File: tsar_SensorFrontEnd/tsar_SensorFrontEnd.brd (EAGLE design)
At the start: 128.5 x 85.1 mm, 217 parts, among them U1 ADS8344N, U2 ADS8344N

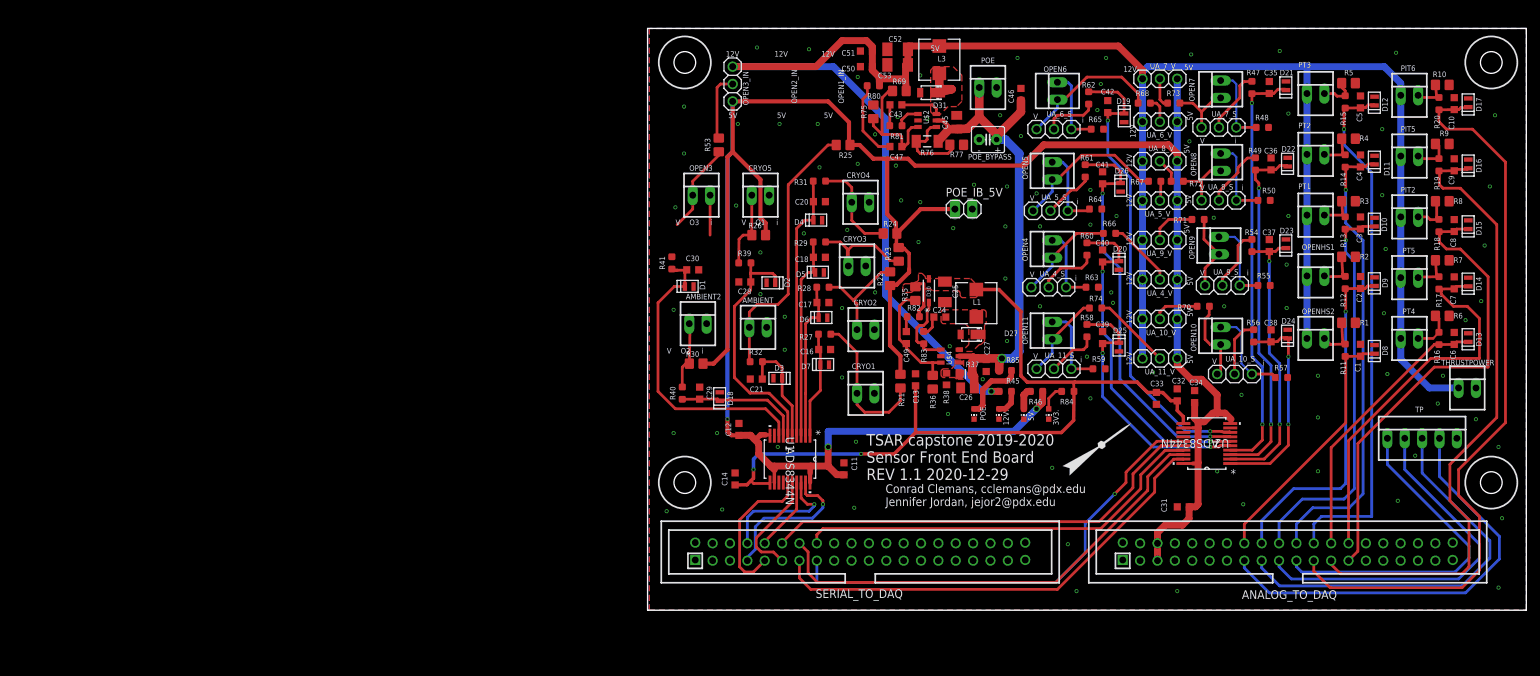
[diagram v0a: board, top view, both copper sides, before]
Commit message: POE, SFE changes
POE: added gnd vias and text info
SFE: moved to mar dxf outline. removed unallocated lines and added valve position sensor pinout. updated attributes. the board is currently unrouted.
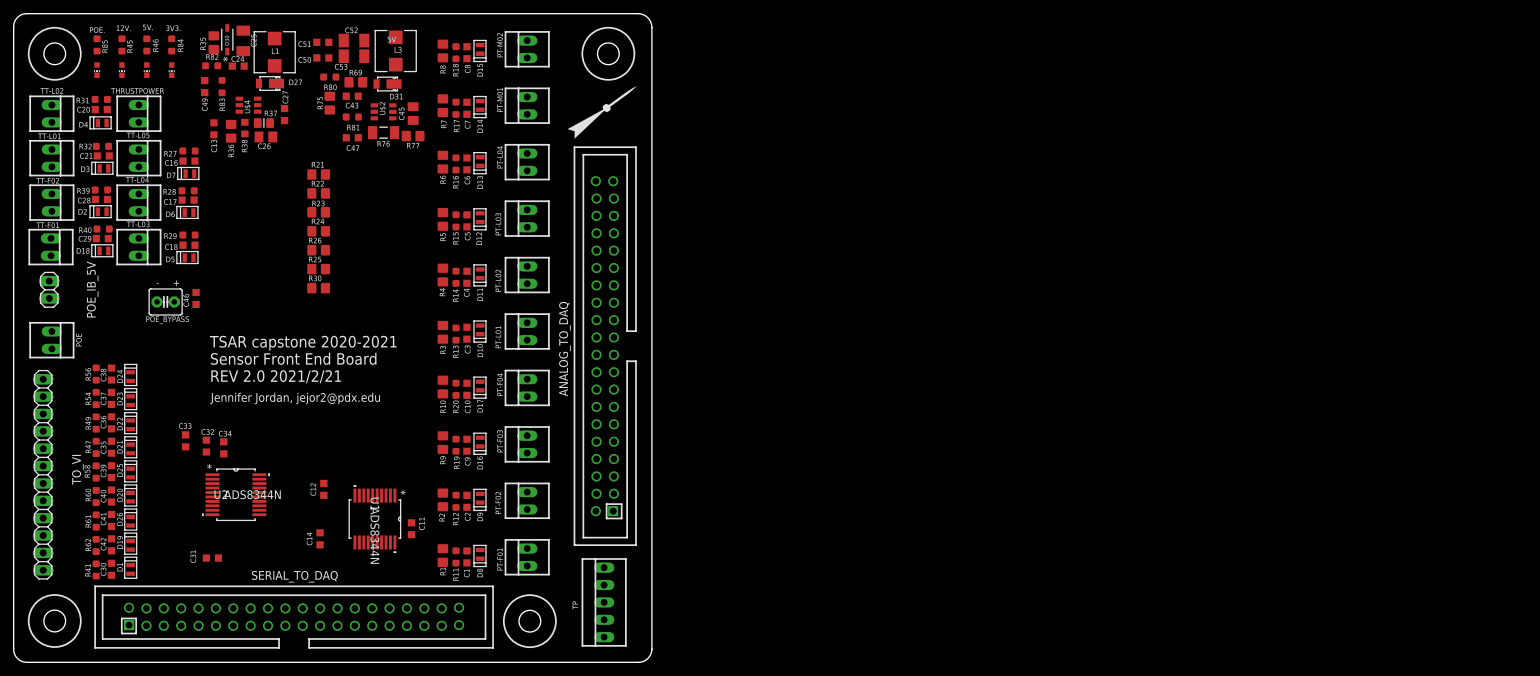
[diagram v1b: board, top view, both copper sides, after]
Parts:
- removed AMBIENT, AMBIENT2, CRYO1, CRYO2, CRYO3, CRYO4, CRYO5, OPEN10, OPEN3, OPEN7, OPEN8, OPEN9, OPENHS1, OPENHS2, PIT2, PIT5, PIT6, PT1, PT2, PT3, PT4, PT5: 22-23-2021, con-molex:22-23-2021
- removed JP3, UA_10_S, UA_10_V, UA_11_S, UA_11_V, UA_4_S, UA_4_V, UA_5_S, UA_5_V, UA_6_S, UA_6_V, UA_7_S, UA_7_V, UA_8_S, UA_8_V, UA_9_S, UA_9_V: (no value), adafruit:1X03
- removed OPEN11, OPEN4, OPEN5, OPEN6: (no value), con-molex:22-23-2021
- removed R48, R50, R55, R57, R59, R63, R64, R65, R66, R67, R68, R70, R71, R72, R73, R74: NP, oresat-rcl:.0603-A-NOSILK
- removed R53: NP, oresat-rcl:.0805-A-NOSILK
- added PT-F01, PT-F02, PT-F03, PT-F04, PT-L01, PT-L02, PT-L03, PT-L04, PT-M01, PT-M02, TT-F01, TT-F02, TT-L01, TT-L02, TT-L03, TT-L04, TT-L05: 22-23-2021, con-molex:22-23-2021
- added TO_VI: (no value), pinhead:1X12
- moved THRUSTPOWER 198.4 mm to (18.3, 80.2), turned to 270 degrees
- moved D21 177.3 mm to (17.0, 31.2), turned to 90 degrees
- moved C35 177.3 mm to (14.3, 31.5), turned to 270 degrees
- moved R47 177.0 mm to (12.1, 31.4), turned to 270 degrees
- moved C36 173.8 mm to (14.3, 35.0), turned to 270 degrees
- moved D22 173.7 mm to (17.0, 34.7), turned to 90 degrees
- moved R49 173.7 mm to (12.1, 35.0), turned to 270 degrees
- moved C37 170.8 mm to (14.3, 38.6), turned to 270 degrees
- moved D23 170.7 mm to (17.0, 38.3), turned to 90 degrees
- moved R54 170.5 mm to (12.1, 38.6), turned to 270 degrees
- moved C38 169.7 mm to (14.3, 42.2), turned to 270 degrees
- moved D24 169.6 mm to (17.0, 41.8), turned to 90 degrees
- moved R56 169.4 mm to (12.1, 42.2), turned to 270 degrees
- moved R62 159.2 mm to (12.1, 17.1)
- moved C42 159.2 mm to (14.3, 17.2), turned to 270 degrees
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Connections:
- removed net N$33: OPEN3.1, R41.2, R53.1
- removed net N$36: JP3.2, R53.2
- removed net N$55: R68.2, UA_6_V.2
- removed net N$57: R67.2, UA_5_V.2
- removed net N$58: R66.2, UA_4_V.2
- removed net N$59: OPEN4.2, R63.2, UA_4_S.3
- removed net N$60: OPEN5.2, R64.2, UA_5_S.3
- removed net N$61: OPEN6.2, R65.2, UA_6_S.3
- removed net N$62: OPEN6.1, R68.1, UA_6_S.1
- removed net N$63: OPEN5.1, R67.1, UA_5_S.1
- removed net N$64: OPEN4.1, R66.1, UA_4_S.1
- removed net N$65: OPEN7.2, R48.2, UA_7_S.3
- removed net N$66: OPEN7.1, R73.1, UA_7_S.1
- removed net N$67: R47.2, UA_7_S.2
- removed net N$68: R60.2, UA_4_S.2
- removed net N$69: R61.2, UA_5_S.2
- removed net N$70: R62.2, UA_6_S.2
- removed net N$71: OPEN8.2, R50.2, UA_8_S.3
- removed net N$72: OPEN8.1, R72.1, UA_8_S.1
- removed net N$73: R49.2, UA_8_S.2
- removed net N$74: OPEN9.2, R55.2, UA_9_S.3
- removed net N$75: OPEN9.1, R71.1, UA_9_S.1
- removed net N$76: R54.2, UA_9_S.2
- removed net N$77: OPEN10.2, R57.2, UA_10_S.3
- removed net N$78: OPEN10.1, R70.1, UA_10_S.1
- removed net N$79: R56.2, UA_10_S.2
- removed net N$80: OPEN11.2, R59.2, UA_11_S.3
- removed net N$81: OPEN11.1, R74.1, UA_11_S.1
- removed net N$82: R58.2, UA_11_S.2
- removed net N$87: R71.2, UA_9_V.2
- removed net N$88: R70.2, UA_10_V.2
- removed net N$93: R74.2, UA_11_V.2
- removed net N$94: R73.2, UA_7_V.2
- removed net N$95: R72.2, UA_8_V.2
- new net HES1: R56.2, TO_VI.1
- new net HES2: R54.2, TO_VI.2
- new net HES3: R49.2, TO_VI.3
- new net HES4: R47.2, TO_VI.4
- new net HES5: R58.2, TO_VI.5
- new net HES6: R60.2, TO_VI.6
- new net HES7: R61.2, TO_VI.7
- new net HES8: R62.2, TO_VI.8
- new net HES9: R41.2, TO_VI.9
- net +12V: now also PT-F01.1, PT-F02.1, PT-F03.1, PT-F04.1, PT-L01.1, PT-L02.1, PT-L03.1, PT-L04.1, PT-M01.1, PT-M02.1; no longer JP3.1, OPENHS1.1, OPENHS2.1, PIT2.1, PIT5.1, PIT6.1, PT1.1, PT2.1, PT3.1, PT4.1, PT5.1, UA_10_V.3, UA_11_V.3, UA_4_V.3, UA_5_V.3, UA_6_V.3, UA_7_V.3, UA_8_V.3, UA_9_V.3
- net +5V: no longer JP3.3, UA_10_V.1, UA_11_V.1, UA_4_V.1, UA_5_V.1, UA_6_V.1, UA_7_V.1, UA_8_V.1, UA_9_V.1
- net AMBIENT: now also R26.1, TT-L01.1; no longer AMBIENT.1, R25.1
- net CRYO1: now also TT-L05.1; no longer CRYO1.1
- net CRYO2: now also TT-L04.1; no longer CRYO2.1
- net CRYO3: now also TT-L03.1; no longer CRYO3.1
- net CRYO4: now also TT-L02.1; no longer CRYO4.1
- net GND: now also TT-F01.2, TT-F02.2, TT-L01.2, TT-L02.2, TT-L03.2, TT-L04.2, TT-L05.2; no longer AMBIENT.2, AMBIENT2.2, CRYO1.2, CRYO2.2, CRYO3.2, CRYO4.2, CRYO5.2, OPEN3.2, R48.1, R50.1, R55.1, R57.1, R59.1, R63.1, R64.1, R65.1
- net N$1: now also PT-L02.2; no longer PT2.2
- net N$19: now also PT-F01.2; no longer OPENHS2.2
- net N$2: now also PT-F02.2; no longer OPENHS1.2
- net N$22: now also PT-L01.2; no longer PT1.2
- net N$29: now also PT-L03.2; no longer PT3.2
- net N$32: now also R25.1, TT-F02.1; no longer CRYO5.1, R26.1
- net N$34: now also TT-F01.1; no longer AMBIENT2.1
- net N$38: now also PT-L04.2; no longer PT4.2
- net N$40: now also PT-M01.2; no longer PT5.2
- net N$46: now also PT-F04.2; no longer PIT6.2
- net N$6: now also PT-M02.2; no longer PIT2.2
- net N$7: now also PT-F03.2; no longer PIT5.2
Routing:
- net +5V: track 382.6 -> 0.00 mm, vias 3 -> 0
- net +12V: track 321.5 -> 0.00 mm, vias 1 -> 0
- net +3V3: track 122.4 -> 0.00 mm, vias 2 -> 0
- net ADC0.4: track 110.0 -> 0.00 mm
- net ADC0.5: track 93.1 -> 0.00 mm
- net ADC1.4: track 77.8 -> 0.00 mm, vias 1 -> 0
- net +24V: track 76.1 -> 0.00 mm, vias 1 -> 0
- net ADC0.6: track 69.8 -> 0.00 mm
- net DIO39/SPI1-NSS: track 69.2 -> 0.00 mm
- net DIO40/SPI1-MISO: track 68.8 -> 0.00 mm, vias 1 -> 0
- net DIO40/SPI1-SCK: track 68.5 -> 0.00 mm
- net 17: track 68.1 -> 0.00 mm, vias 2 -> 0
- net ADC1.3: track 67.7 -> 0.00 mm, vias 1 -> 0
- net DIO37: track 65.9 -> 0.00 mm
- net ADC0.0: track 63.2 -> 0.00 mm
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- removed copper zone on layer 1, net +3V3
- removed copper zone on layer 1, net FLY1
- removed copper zone on layer 1, net FLY3
- removed copper zone on layer 1, net GND
- removed copper zone on layer 16, net GND
- removed copper zone on layer 1, net N$8
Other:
- board size 128.5 x 85.1 mm -> 93.3 x 94.9 mm
- board text added: "Jennifer Jordan, jejor2@pdx.edu"
- board text added: "TSAR capstone 2020-2021 Sensor Front End Board REV 2.0 2021/2/21"
- board text removed: "12V"
- board text removed: "Conrad Clemans, cclemans@pdx.edu Jennifer Jordan, jejor2@pdx.edu"
- board text removed: "O1"
- board text removed: "O2"
- board text removed: "O3"
- board text removed: "OPEN1_IN"
- board text removed: "OPEN2_IN"
- board text removed: "OPEN3_IN"
- board text removed: "TSAR capstone 2019-2020 Sensor Front End Board REV 1.1 2020-12-29"
- board text removed: "V"
- board text removed: "i"
